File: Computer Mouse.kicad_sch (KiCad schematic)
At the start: 37 parts, among them J1 USB_C_Receptacle_USB2.0, J2 Conn_01x02, Q1 MMDT3906, Q2 MMDT3906, Q3 MMDT3906, Q4 MMDT3906, SW1 SW_SPDT, SW2 SW_SPDT, SW3 SW_SPDT, SW4 SW_SPDT, SW5 SW_SPST, SW6 RotaryEncoder, SW7 RotaryEncoder, U2 MCP73831-2-OT, U3 STM32F103RCT6

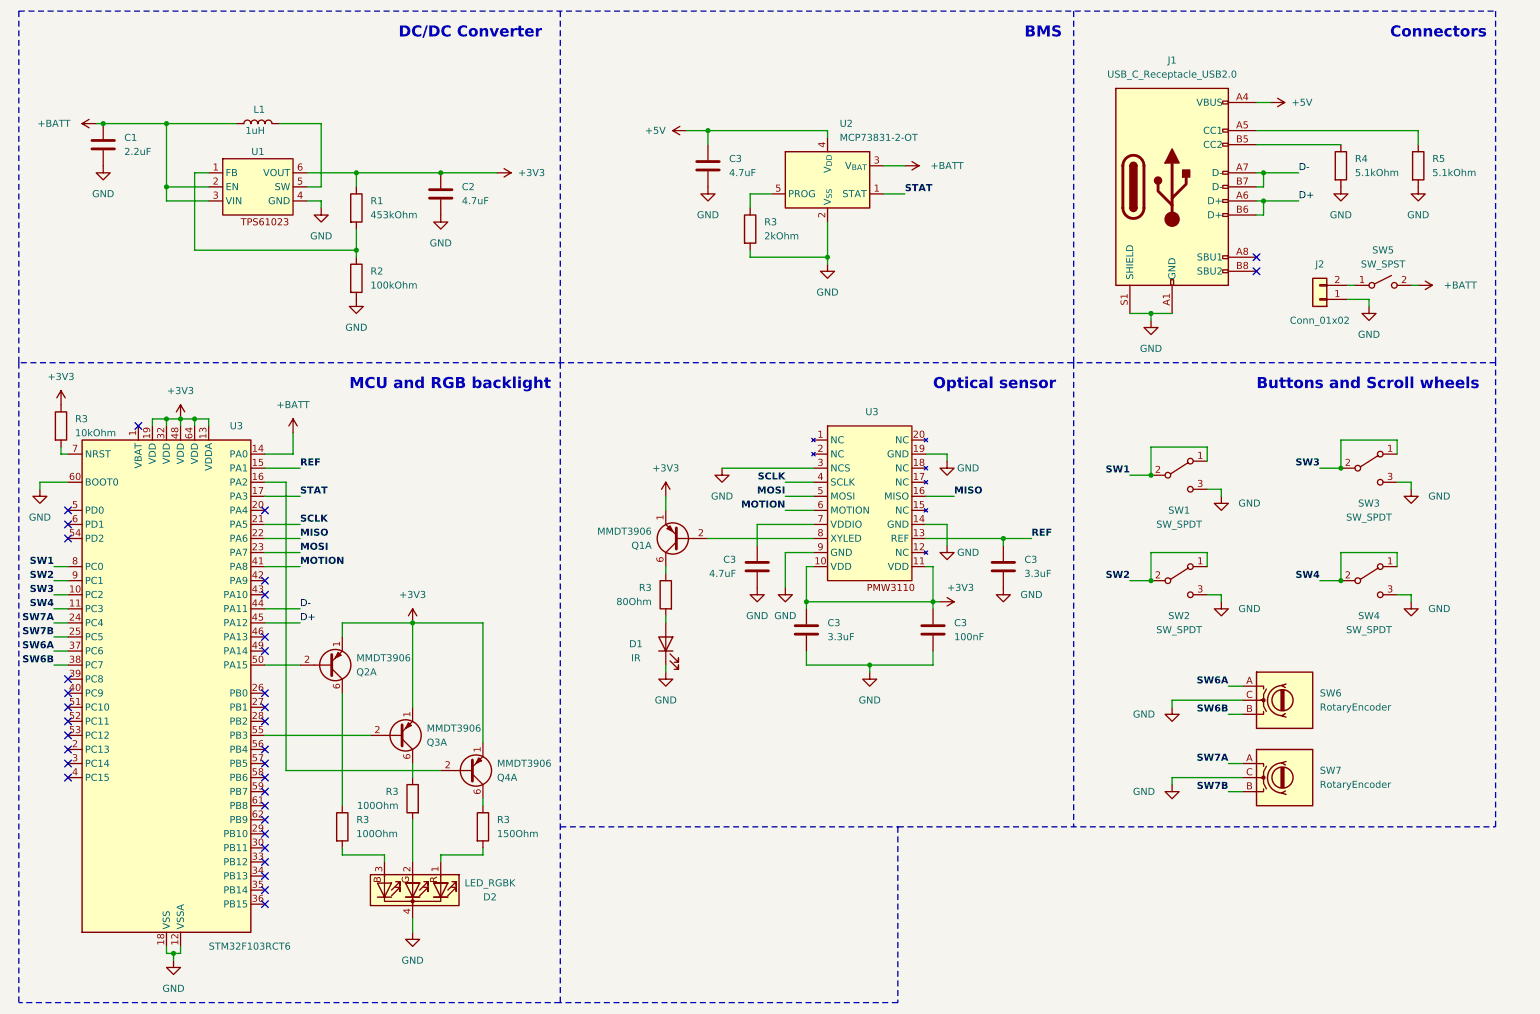
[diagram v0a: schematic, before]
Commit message: BT module
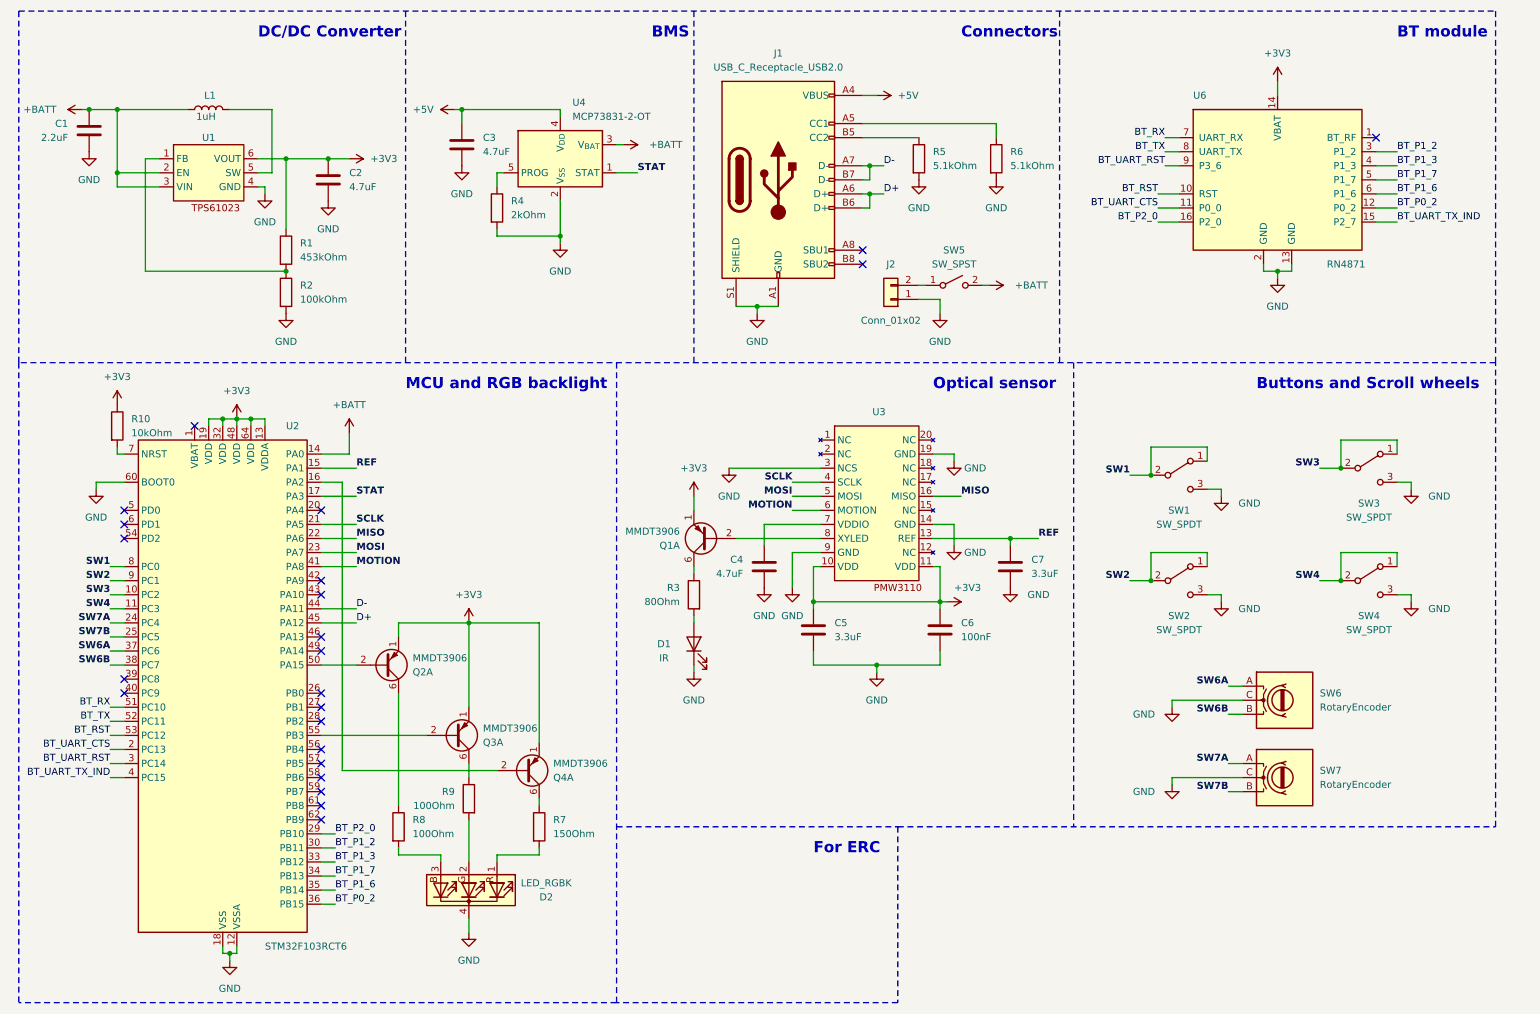
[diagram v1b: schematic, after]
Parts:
- added U6: RN4871, RF_Module:ST_SPBTLE, symbol RF_Bluetooth:RN4871
- J1: footprint (none) -> Connector_USB:USB_C_Receptacle_GCT_USB4085
- J2: footprint (none) -> Connector_JST:JST_EH_B2B-EH-A_1x02_P2.50mm_Vertical
- renumbered C3 to C4, C3 to C5, C3 to C6, C3 to C7, R3 to R10, R3 to R4, R4 to R5, R5 to R6, R3 to R7, R3 to R8, R3 to R9, U3 to U2, U2 to U4
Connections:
- net +3V3: now also U6.14 (VBAT)
- net GND: now also U6.13 (GND), U6.2 (GND)
- net BT_UART_CTS: now reaches U2.2 (PC13)
- net BT_UART_CTS: now also U6.11 (P0_0)
- net BT_P2_0: now reaches U2.29 (PB10)
- net BT_P2_0: now also U6.16 (P2_0)
- net BT_UART_RST: now reaches U2.3 (PC14)
- net BT_UART_RST: now also U6.9 (P3_6)
- net BT_P1_2: now reaches U2.30 (PB11)
- net BT_P1_2: now also U6.3 (P1_2)
- net BT_P1_3: now reaches U2.33 (PB12)
- net BT_P1_3: now also U6.4 (P1_3)
- net BT_P1_7: now reaches U2.34 (PB13)
- net BT_P1_7: now also U6.5 (P1_7)
- net BT_P1_6: now reaches U2.35 (PB14)
- net BT_P1_6: now also U6.6 (P1_6)
- net BT_P0_2: now reaches U2.36 (PB15)
- net BT_P0_2: now also U6.12 (P0_2)
- net BT_UART_TX_IND: now reaches U2.4 (PC15)
- net BT_UART_TX_IND: now also U6.15 (P2_7)
- net BT_RX: now reaches U2.51 (PC10)
- net BT_RX: now also U6.7 (UART_RX)
- net BT_TX: now reaches U2.52 (PC11)
- net BT_TX: now also U6.8 (UART_TX)
- net BT_RST: now reaches U2.53 (PC12)
- net BT_RST: now also U6.10 (RST)
- no-connect marks 34 -> 23
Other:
- note added: "BT module"
- note added: "For ERC"
- moved on the sheet: C1, C2, C3, C4, C5, C6, C7, D1, D2, J1, J2, L1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
